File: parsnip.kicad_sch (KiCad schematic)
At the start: 69 parts, among them J1 SPI BUS, J2 I2C3, J3 I2C1, J4 I2C2, J5 e-Ink Display Connector, J6 UART0, SW1 ESP_RESET, SW2 BOOT, U1 ESP32-S3-WROOM-1-N16R8, Y1 32.768KHz

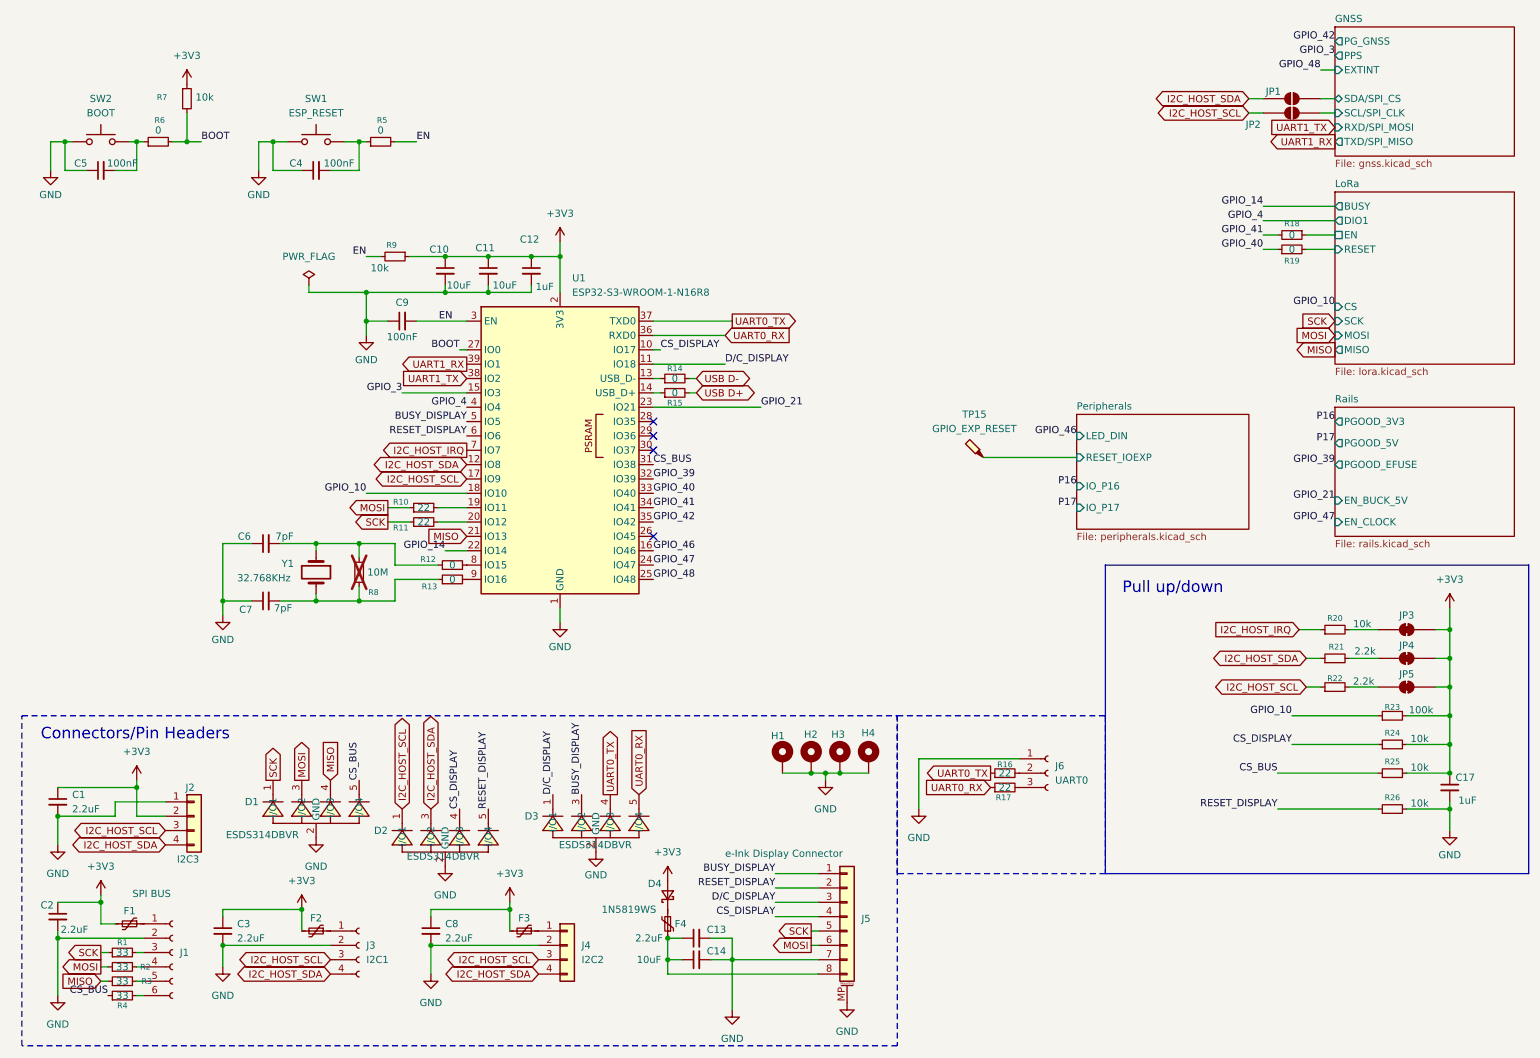
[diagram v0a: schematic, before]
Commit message: progress in layout!
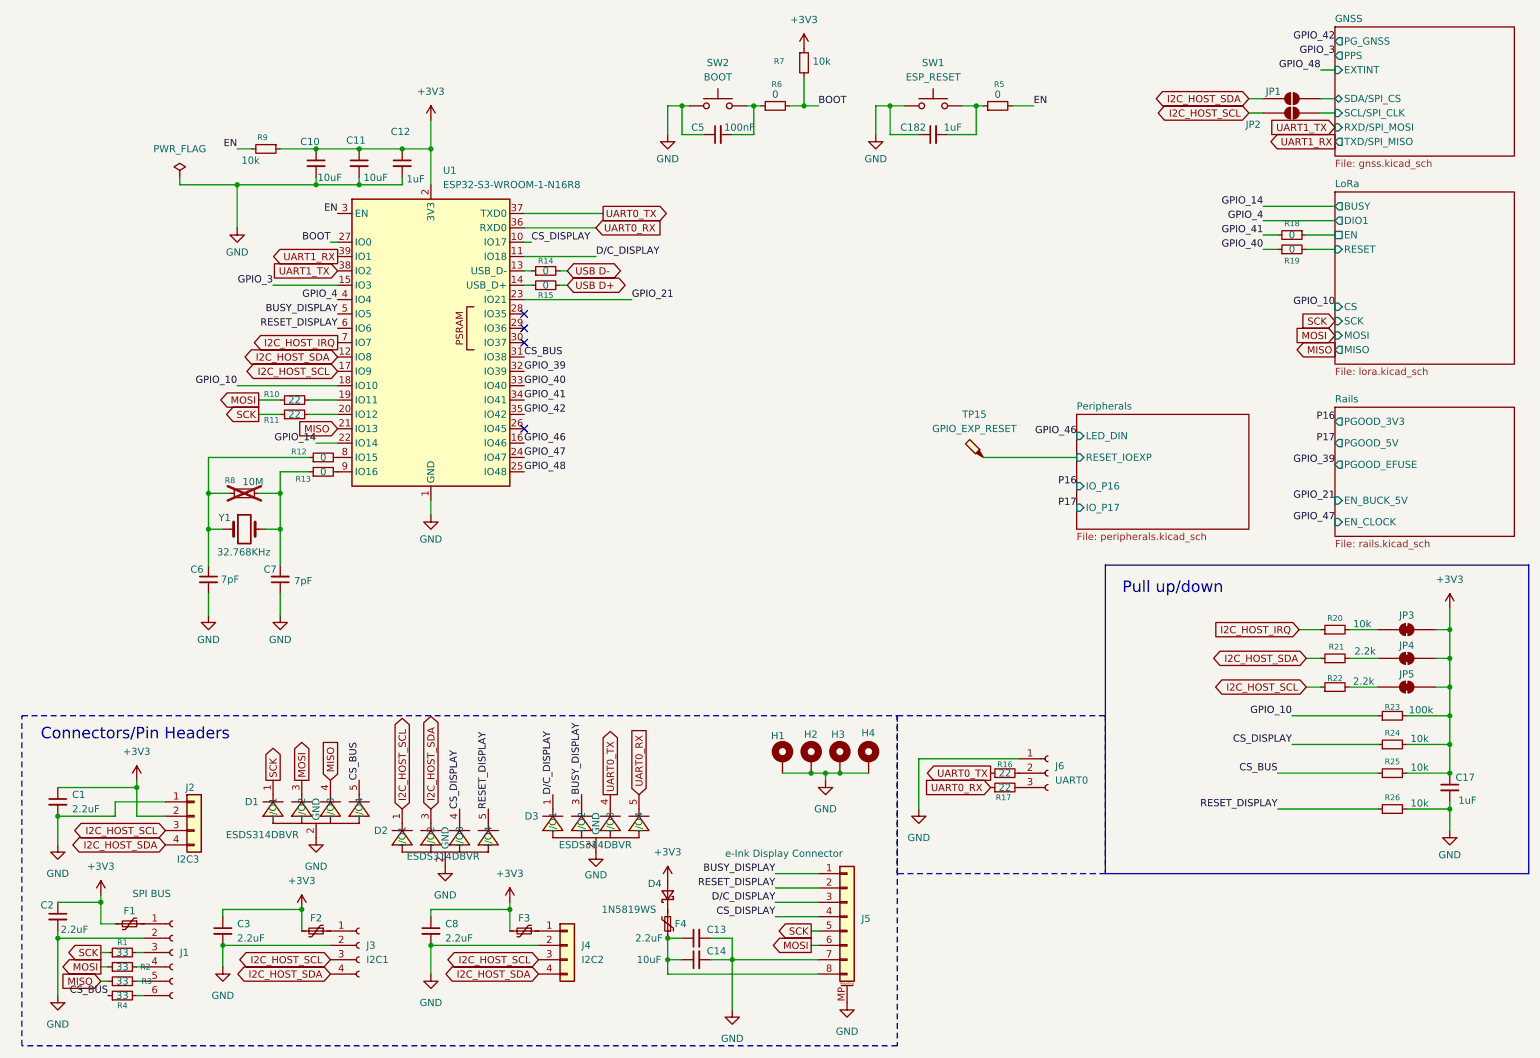
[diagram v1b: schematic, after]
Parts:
- removed C4, C9: 100nF, Capacitor_SMD:C_0402_1005Metric, symbol Device:C_Small
- added C182: 1uF, Capacitor_SMD:C_0402_1005Metric, symbol Device:C_Small
- TP15: footprint TestPoint:TestPoint_Pad_D1.0mm -> TestPoint:TestPoint_Pad_D1.5mm
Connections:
- net GND: now also C6.2, C182.1; no longer C6.1
- net at R12.1, R8.2, Y1.1: now also C6.1; no longer C6.2
- net at R5.1, SW1.2: now also C182.2
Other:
- moved on the sheet: C10, C11, C12, C5, R10, R11, R12, R13, R14, R15, R5, R6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
